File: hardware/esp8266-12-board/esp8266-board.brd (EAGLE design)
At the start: 33.5 x 38.1 mm, 24 parts, among them T1 AMS1117, T2 LM7805

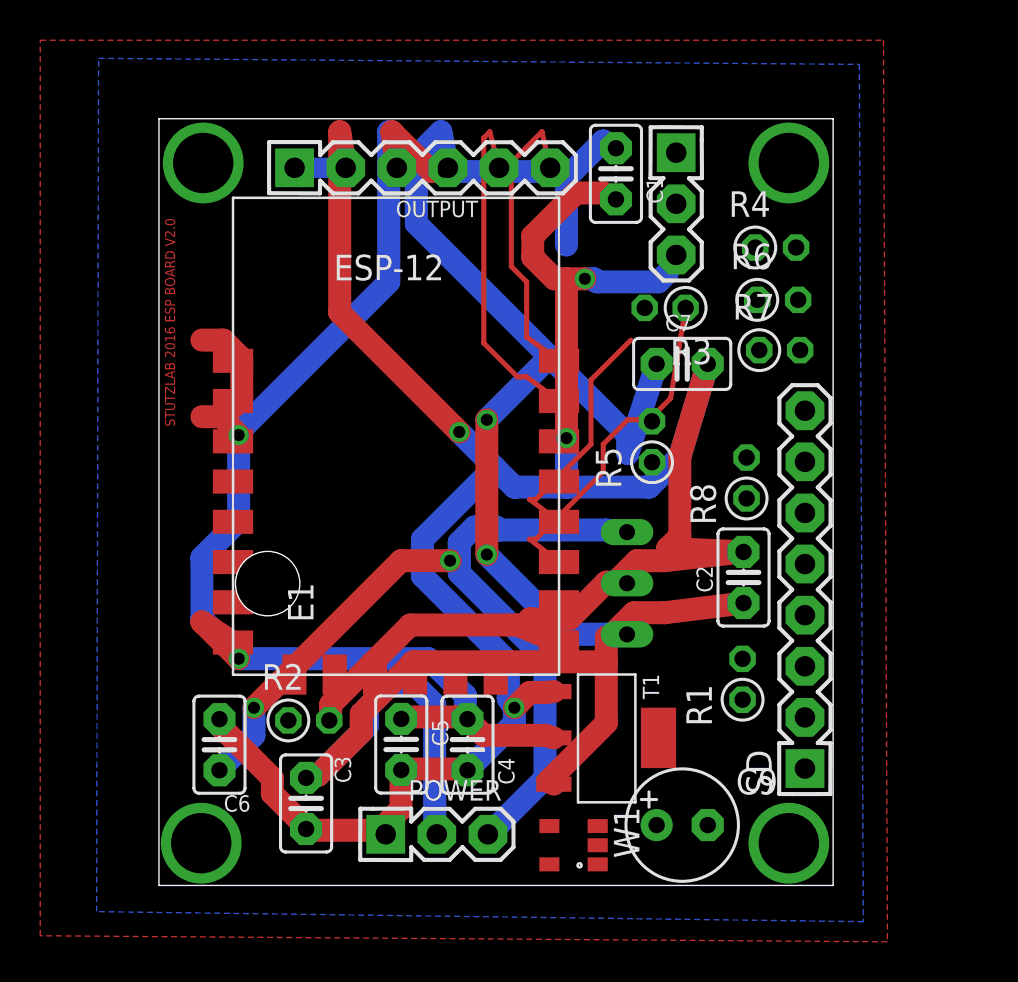
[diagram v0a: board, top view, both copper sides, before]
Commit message: commit
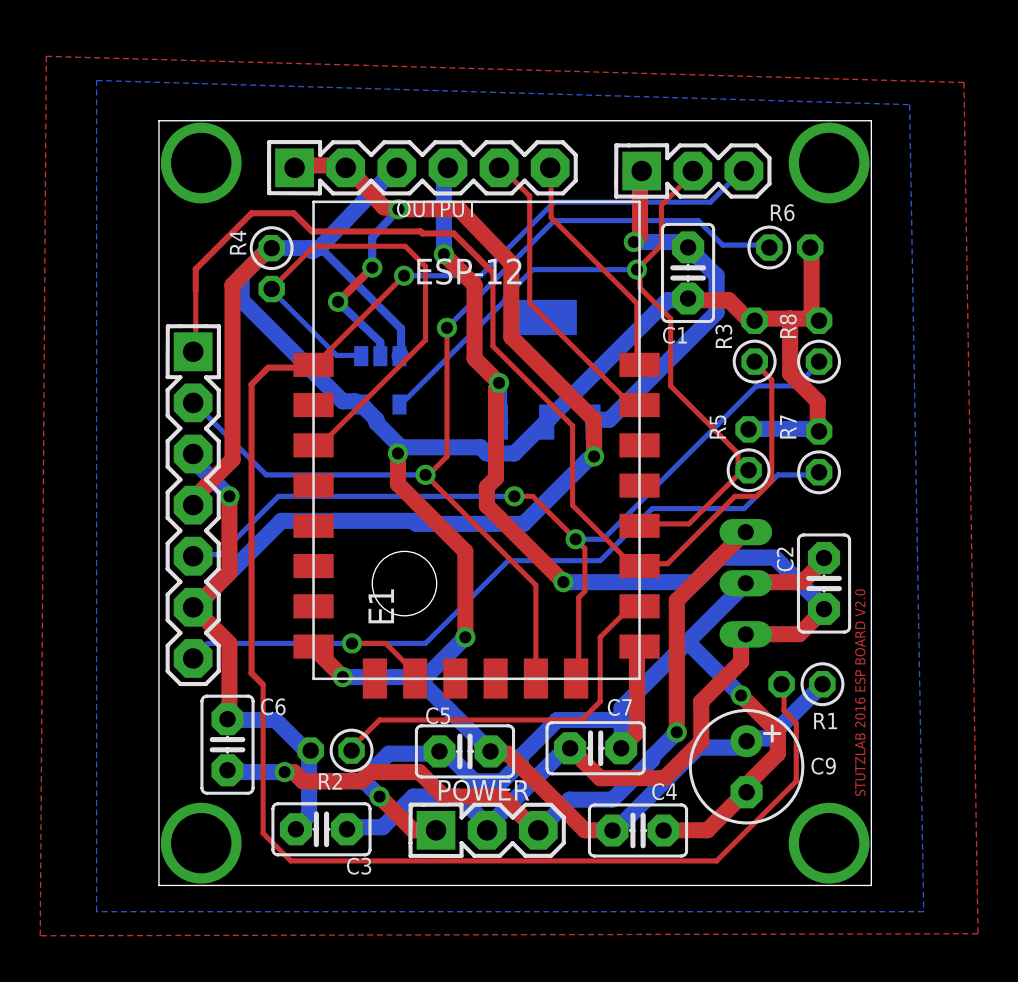
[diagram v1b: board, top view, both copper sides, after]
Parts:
- removed SD: PIN-HEADER-8PIN, stutz-eagle:PIN-HEADER-8PIN
- added SD1: CS SI GND 3.3V SCK GND SO, stutz-eagle:PIN-HEADER-7PIN
- FIRMWARE: value FIRMWARE -> GND DTR RTS
- OUTPUT: value GND GND 3.3V 5V RX TX -> GND GND 3.3V 5V RX TX
- moved R4 25.3 mm to (5.60, 30.4), turned to 270 degrees
- moved W1 25.1 mm to (11.0, 25.2), flipped to the bottom, turned to 0 degrees
- moved C7 19.6 mm to (21.7, 6.82)
- moved T1 18.5 mm to (19.3, 25.6), flipped to the bottom, turned to 0 degrees
- moved C4 9.49 mm to (23.8, 2.73), turned to 0 degrees
- moved R8 7.69 mm to (32.8, 27.3)
- moved C1 6.09 mm to (26.3, 30.4), turned to 90 degrees
- moved T2 5.90 mm to (20.3, 15.0)
- moved R7 5.09 mm to (32.8, 21.8), turned to 90 degrees
- moved R3 4.90 mm to (29.6, 27.3), turned to 90 degrees
- moved R5 4.82 mm to (29.3, 21.9)
- moved C9 4.32 mm to (29.2, 5.90), turned to 270 degrees
- moved C2 4.01 mm to (33.0, 15.0)
- moved E1 4.00 mm to (15.3, 21.3)
- moved C5 3.19 mm to (15.2, 6.66), turned to 180 degrees
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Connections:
- removed net SD_NC: SD.1
- net +3.3V: now also SD1.4; no longer SD.5
- net ESP_GPIO2: now also SD1.1; no longer SD.2
- net GND: now also SD1.3, SD1.6; no longer SD.4, SD.7
- net SD_MISO: now also SD1.7; no longer SD.8
- net SD_MOSI: now also SD1.2; no longer SD.3
- net SD_SCK: now also SD1.5; no longer SD.6
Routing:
- net ESP_RST: track 0.00 -> 85.3 mm, vias 0 -> 1
- net SD_MOSI: track 0.00 -> 52.1 mm, vias 0 -> 2
- net SD_SCK: track 0.00 -> 44.2 mm, vias 0 -> 2
- net +3.3V: track 84.2 -> 128.2 mm
- net SD_MISO: track 0.00 -> 39.0 mm, vias 0 -> 1
- net ESP_GPIO2: track 17.1 -> 53.7 mm
- net ESP_GPIO0: track 12.0 -> 40.2 mm, vias 0 -> 1
- net ESP_CH_PD: track 0.00 -> 26.2 mm
- net +5V: track 97.4 -> 73.1 mm, vias 2 -> 3
- net ESP_GPIO15: track 0.00 -> 19.2 mm
- net GND: track 144.8 -> 160.0 mm, vias 4 -> 8
- net +24V: track 43.2 -> 37.4 mm
- net ESP_TX: track 15.0 -> 11.7 mm
- net ESP_RX: track 17.3 -> 15.0 mm
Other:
- board size 33.5 x 38.1 mm -> 35.4 x 38 mm
